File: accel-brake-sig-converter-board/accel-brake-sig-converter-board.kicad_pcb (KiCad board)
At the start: 2 copper layers, 30 x 90 mm, 89 parts, among them J1 SM03B-PASS-TBT, J2 SM03B-PASS-TBT, J3 SM03B-PASS-TBT, J4 SM03B-PASS-TBT, J5 SM03B-PASS-TBT, J6 SM03B-PASS-TBT, Q1 DMP3098LQ-7, Q2 DMP3098LQ-7, Q3 DMP3098LQ-7, Q4 2N7002K-AU_R1_000A2, Q5 2N7002K-AU_R1_000A2, Q6 2N7002K-AU_R1_000A2, U1 NCV8711BMTW500TBG, U2 NCV8711BMTW500TBG, U3 NCV8711BMTW500TBG, U4 NCV20072DR2G, U5 NCV20072DR2G, U6 NCV20072DR2G

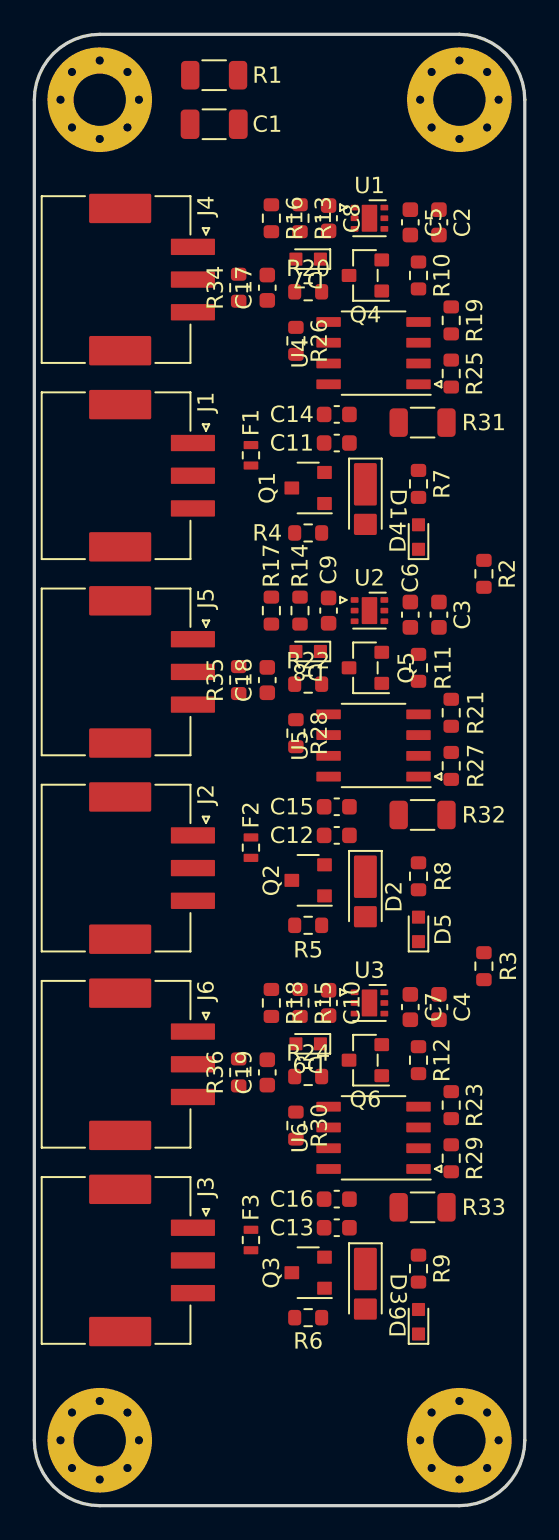
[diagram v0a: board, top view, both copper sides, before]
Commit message: 配置完了
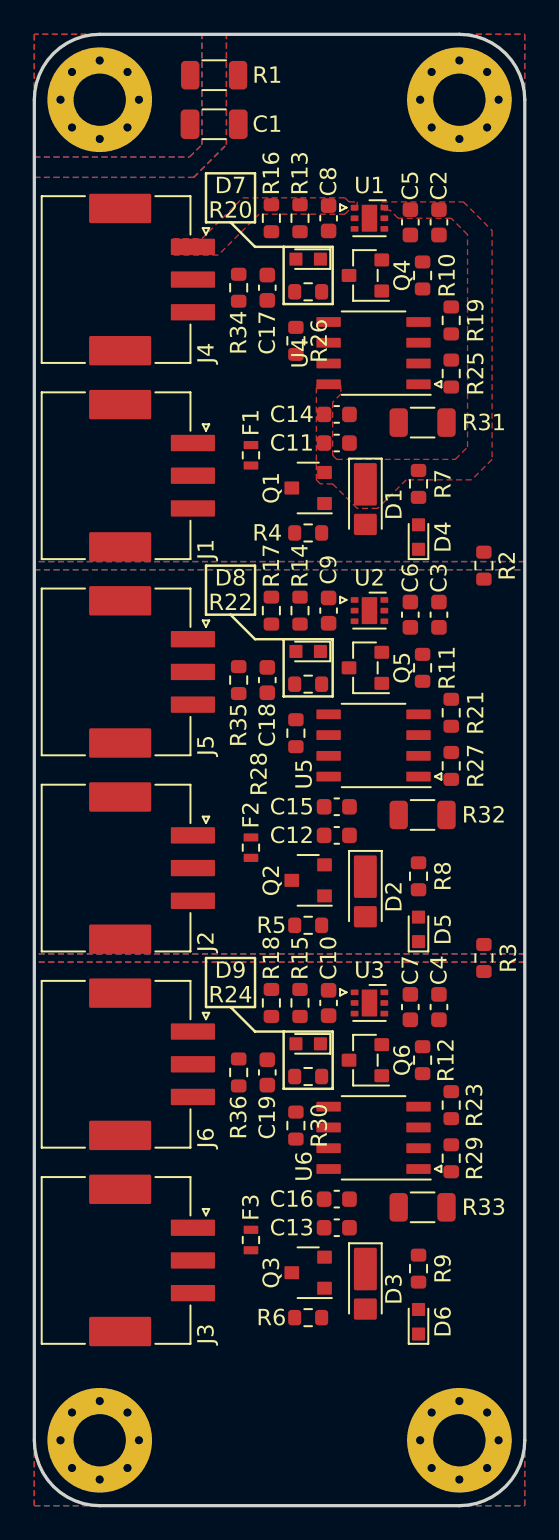
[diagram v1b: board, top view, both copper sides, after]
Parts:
- moved R2 0.50 mm to (27.5, 32.5)
- moved R3 0.50 mm to (27.5, 56.5)
- moved R10 0.25 mm to (23.8, 14.8)
- moved R11 0.25 mm to (23.8, 38.8)
- moved R12 0.25 mm to (23.8, 62.8)
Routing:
- added copper zone on F.Cu, net +12V1
- added copper zone on B.Cu, net Chassis
- added copper zone on F.Cu, net Chassis
- added copper zone on B.Cu, net GND1
- added copper zone on F.Cu, net GND1
- added copper zone on B.Cu, net GND2
- added copper zone on F.Cu, net GND2
- added copper zone on B.Cu, net GND3
- added copper zone on F.Cu, net GND3
- added copper zone on F.Cu, net VCC1

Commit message: accel1配線
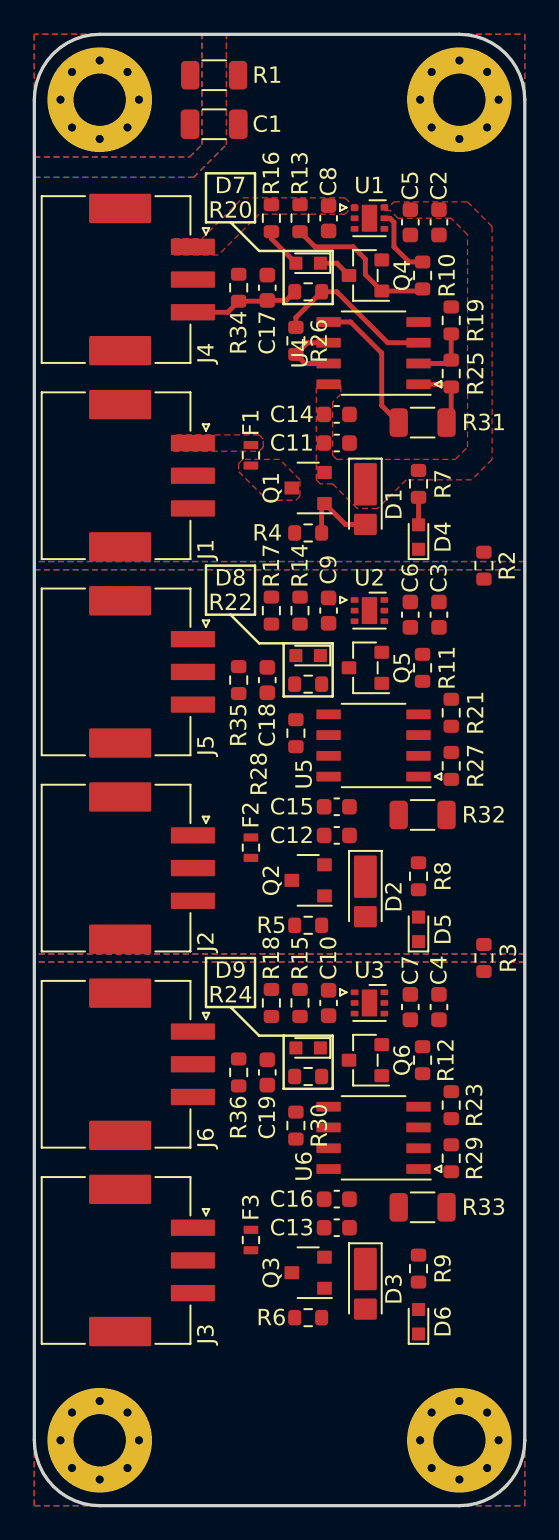
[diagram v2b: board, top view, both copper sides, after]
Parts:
- moved D7 0.25 mm to (16.8, 14.0)
- moved D8 0.25 mm to (16.8, 38.0)
- moved D9 0.25 mm to (16.8, 62.0)
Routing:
- net Net-(U4A-+): track 0.00 -> 10.0 mm
- net Net-(Q4-G): track 0.00 -> 9.61 mm
- net ACCEL1_SIG_OUT_I: track 0.00 -> 8.72 mm
- net ACCEL1_SIG_IN_V: track 0.00 -> 6.74 mm
- net Net-(D1-A): track 0.00 -> 4.90 mm
- net Net-(U4B--): track 0.00 -> 4.53 mm
- net Net-(R25-Pad2): track 0.00 -> 4.36 mm
- net Net-(U1-PG): track 0.00 -> 4.33 mm
- net Net-(U4A--): track 0.00 -> 3.69 mm
- net Net-(D7-A): track 0.00 -> 2.55 mm
- net Net-(D7-K): track 0.00 -> 2.06 mm
- net Net-(D4-A): track 0.00 -> 1.68 mm
- added copper zone on F.Cu, net Net-(J1-Pin_1)
- added copper zone on F.Cu, net Net-(Q1-D)
